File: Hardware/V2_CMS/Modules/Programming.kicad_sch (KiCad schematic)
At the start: 1 part, among them J10 SPI_Programming

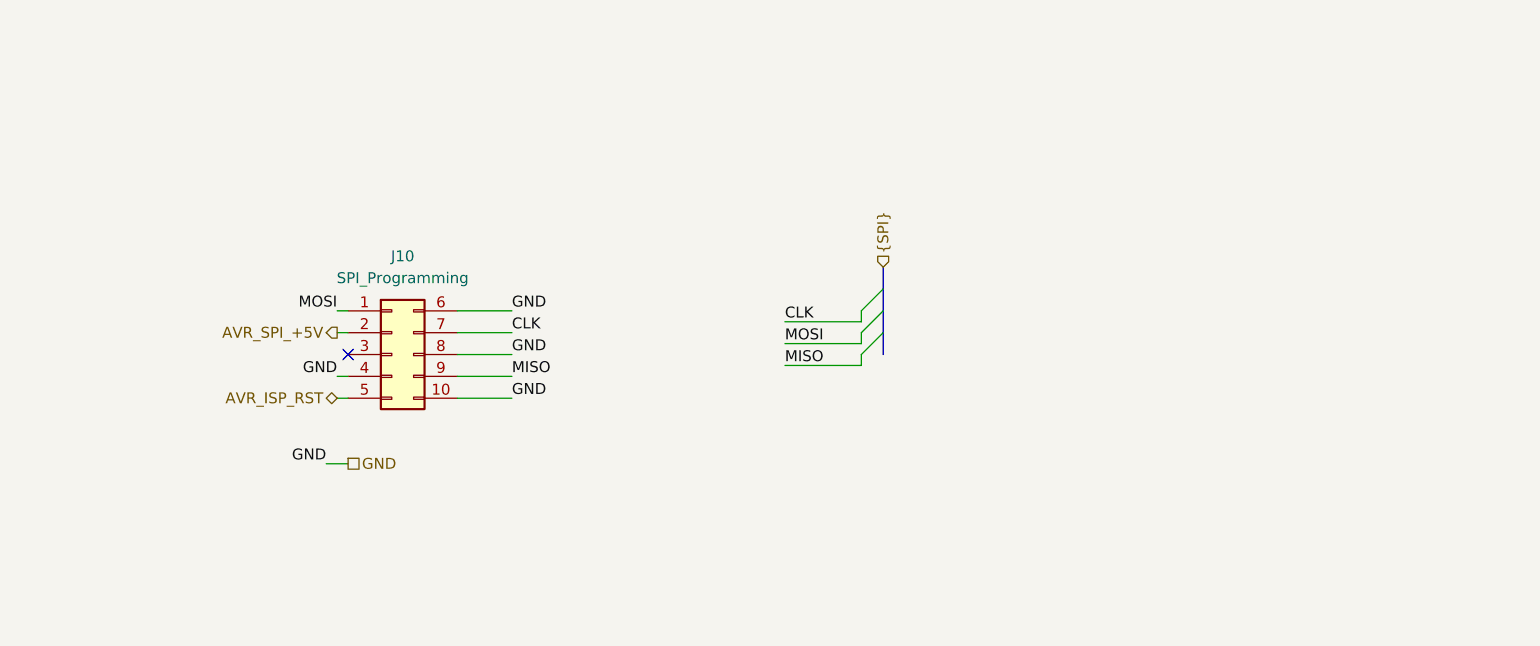
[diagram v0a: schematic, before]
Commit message: update of directory
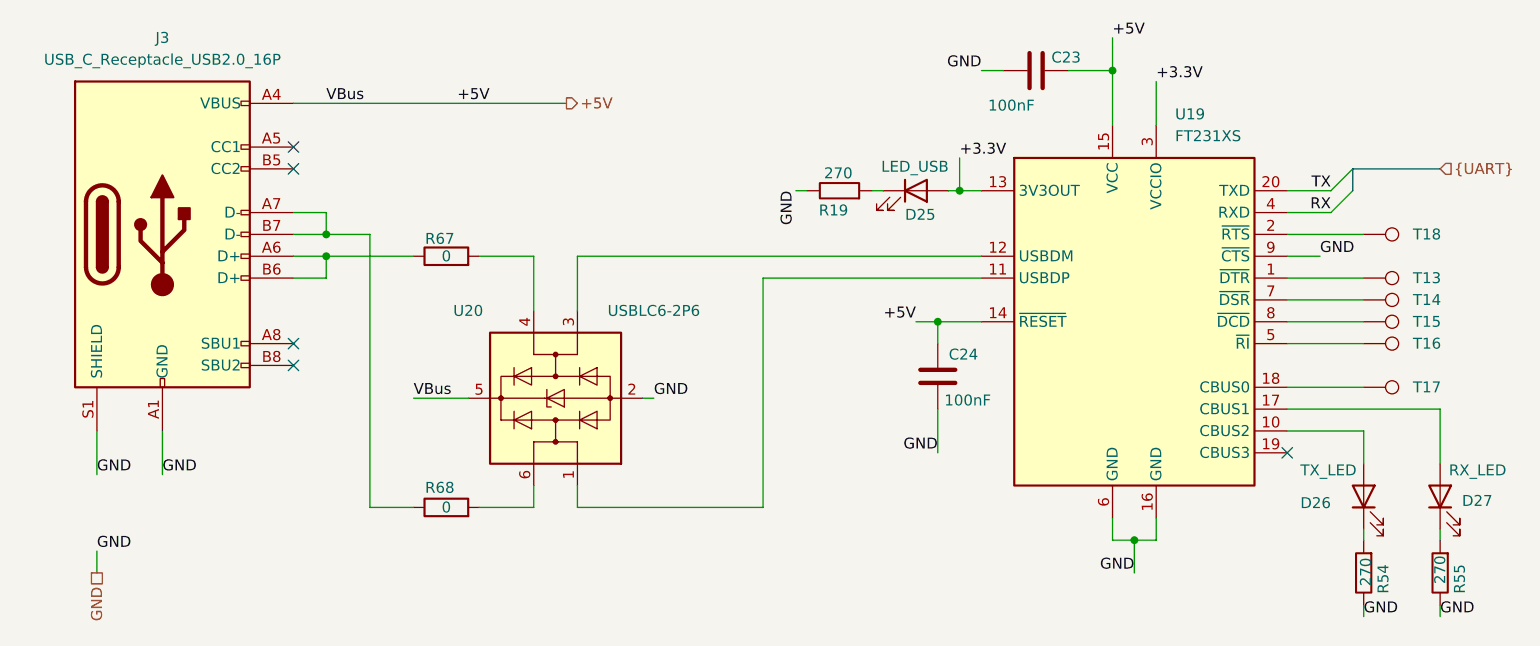
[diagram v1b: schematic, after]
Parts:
- removed J10: SPI_Programming, Connector_PinHeader_2.54mm:PinHeader_2x05_P2.54mm_Vertical, symbol Connector_Generic:Conn_02x05_Top_Bottom
- added C23, C24: 100nF, Capacitor_SMD:C_0603_1608Metric, symbol Device:C
- added D25: LED_USB, LED_SMD:LED_0603_1608Metric, symbol Device:LED
- added D26: TX_LED, LED_SMD:LED_0603_1608Metric, symbol Device:LED
- added D27: RX_LED, LED_SMD:LED_0603_1608Metric, symbol Device:LED
- added J3: USB_C_Receptacle_USB2.0_16P, Connector_USB:USB_C_Receptacle_GCT_USB4085, symbol Connector:USB_C_Receptacle_USB2.0_16P
- added R19, R54, R55: 270, Resistor_SMD:R_0603_1608Metric, symbol PCM_SL_Devices:Resistor_0.5W
- added R67, R68: 0, Resistor_SMD:R_0603_1608Metric, symbol Device:R
- added T13, T14, T15, T16, T17, T18: TP, TestPoint:TestPoint_Pad_D1.0mm, symbol Connector:TestPoint
- added U19: FT231XS, Package_SO:SSOP-20_3.9x8.7mm_P0.635mm, symbol Interface_USB:FT231XS
- added U20: USBLC6-2P6, Package_TO_SOT_SMD:SOT-666, symbol Power_Protection:USBLC6-2P6
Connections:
- net GND: now also C23.2, C24.2, J3.A1 (GND), J3.A12 (GND), J3.B1 (GND), J3.B12 (GND), J3.S1 (SHIELD), R19.2, R54.2, R55.2, U19.16 (GND), U19.6 (GND), U19.9 (~{CTS}), U20.2 (GND)
- new net: D26.1 (K), R54.1
- new net: T18.1, U19.2 (~{RTS})
- new net: D27.1 (K), R55.1
- new net: D27.2 (A), U19.17 (CBUS1)
- new net: J3.A6 (D+), J3.B6 (D+), R67.1
- new net: J3.A7 (D-), J3.B7 (D-), R68.1
- new net: R67.2, U20.4 (I/O2)
- new net: T14.1, U19.7 (~{DSR})
- new net: T15.1, U19.8 (~{DCD})
- new net: T13.1, U19.1 (~{DTR})
- new net: D26.2 (A), U19.10 (CBUS2)
- new net: U19.11 (USBDP), U20.1 (I/O1)
- new net: U19.12 (USBDM), U20.3 (I/O2)
- new net: T17.1, U19.18 (CBUS0)
- new net: T16.1, U19.5 (~{RI})
- new net: D25.1 (K), R19.1
- new net: R68.2, U20.6 (I/O1)
- new net +3.3V: D25.2 (A), U19.13 (3V3OUT), U19.3 (VCCIO)
- new net +5V: C23.1, C24.1, J3.A4 (VBUS), J3.A9 (VBUS), J3.B4 (VBUS), J3.B9 (VBUS), U19.14 (~{RESET}), U19.15 (VCC), U20.5 (VBUS)
- new net RX: U19.4 (RXD)
- new net TX: U19.20 (TXD)
- no-connect marks 1 -> 5
